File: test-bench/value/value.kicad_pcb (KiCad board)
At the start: 2 copper layers, 59.4 x 37.3 mm, 10 parts, among them P1 CONN_02X08, U1 PC817, U2 PC817, U3 PC817

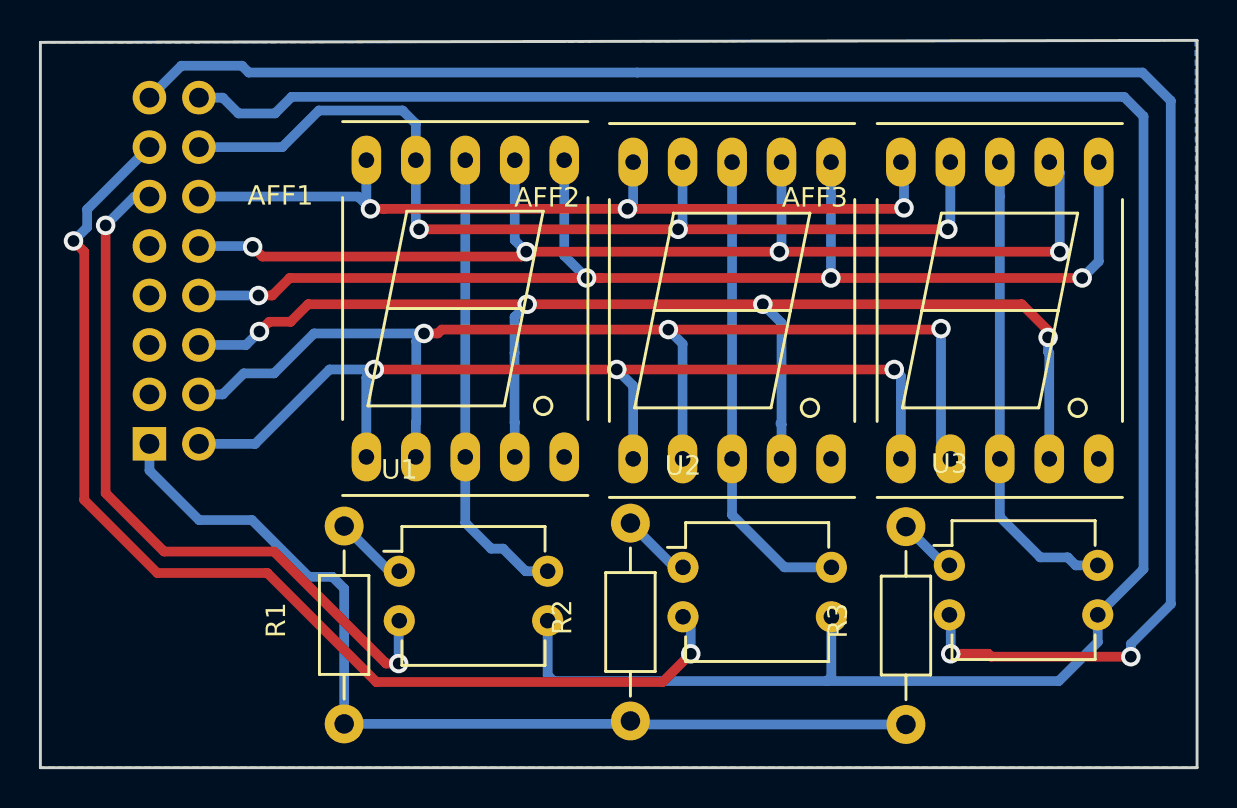
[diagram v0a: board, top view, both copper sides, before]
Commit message: design display beres
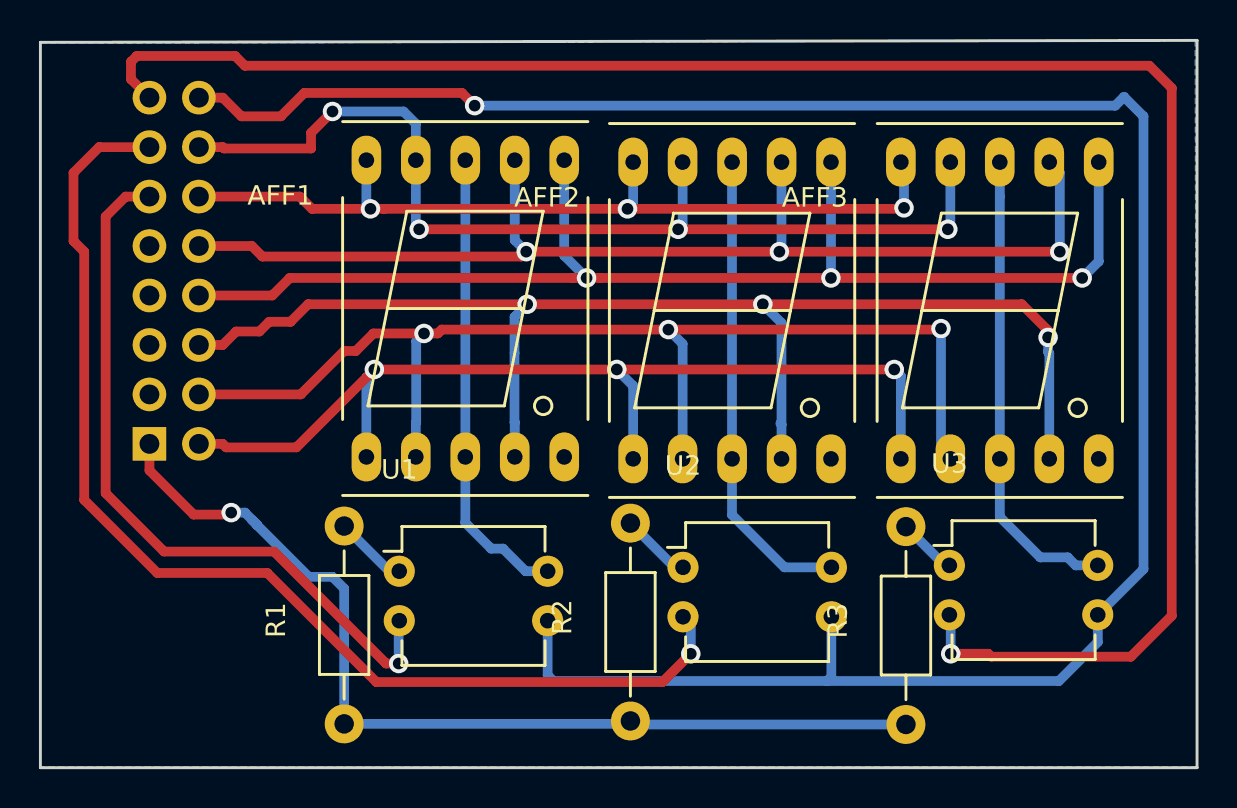
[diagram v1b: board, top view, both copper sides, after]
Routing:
- net /DA: track 94.6 -> 97.9 mm, vias 2 -> 1
- net /DB: track 57.7 -> 59.2 mm, vias 2 -> 1
- net /DC: track 37.5 -> 38.5 mm, vias 2 -> 1
- net GND: track 113.0 -> 113.6 mm, vias 0 -> 1
- net /LF: track 52.1 -> 52.6 mm, vias 3 -> 4
- net VCC: track 50.0 -> 50.5 mm, vias 0 -> 1
- net /LA: vias 4 -> 3
- net /LC: vias 4 -> 3
- net /LB: vias 4 -> 3
